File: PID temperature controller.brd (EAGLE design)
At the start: 82.2 x 72.4 mm, 12 parts, among them IC1 MAX6675

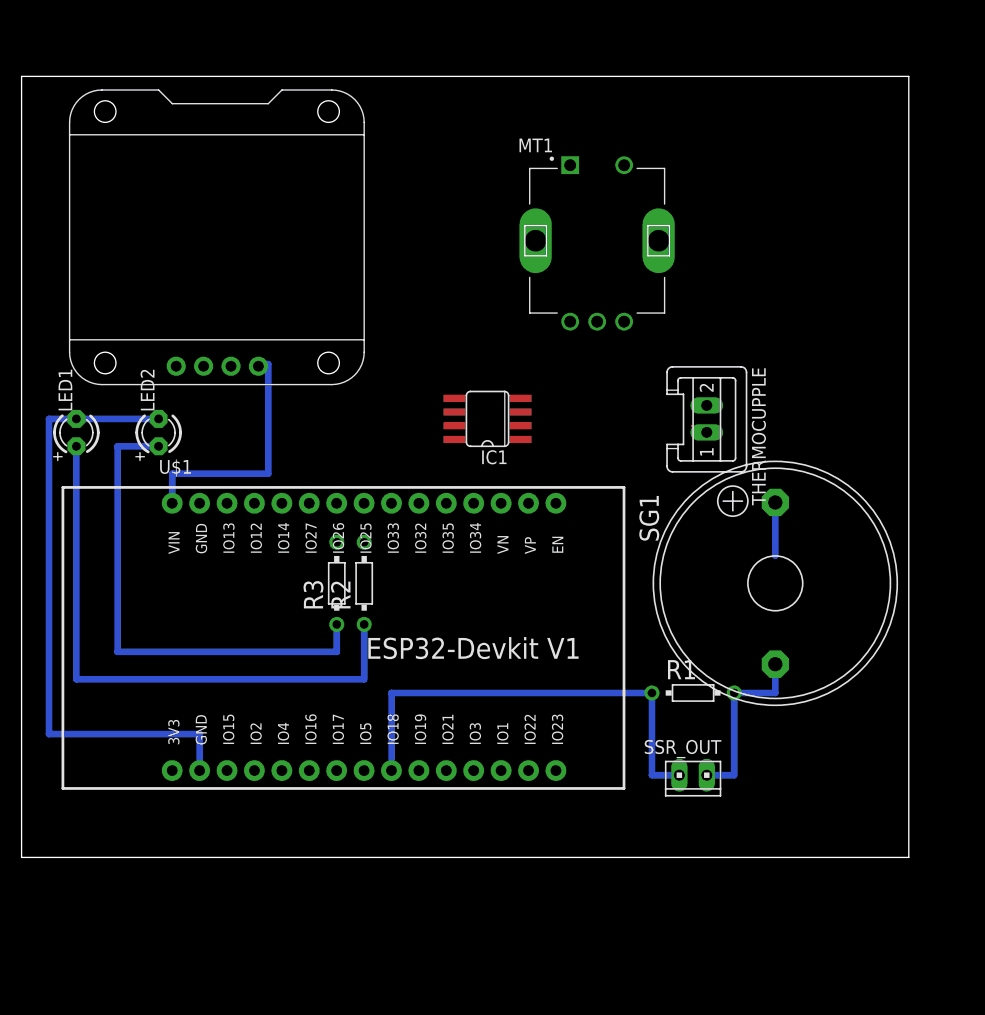
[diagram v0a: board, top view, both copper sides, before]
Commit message: Eagle Schematic and Brd file added
Eagle Schematic and Brd file added
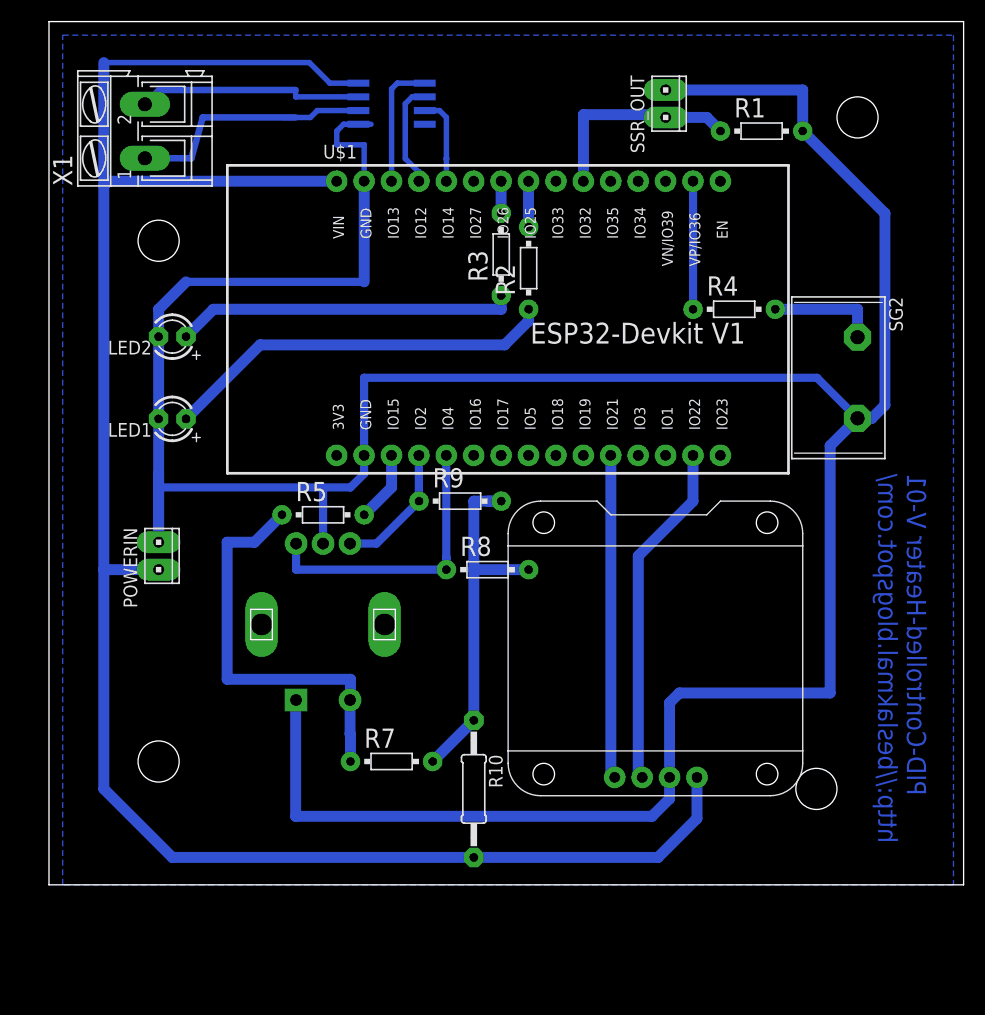
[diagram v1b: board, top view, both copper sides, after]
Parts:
- removed MT1: PEC11R-4215F-S0024, rotary encoder:XDCR_PEC11R-4215F-S0024
- removed SG1: EB2209A, buzzer:EB2209A
- removed THERMOCUPPLE: (no value), con-amp-mt:S02P
- added ENCODER: PEC11R-4215F-S0024, rotary encoder:XDCR_PEC11R-4215F-S0024
- added POWERIN: 5 V, con-amp:10X02MTA
- added R10: 0 Ohm, adafruit:0207/12
- added R4: 100 Ohm, resistor-power:RS1/8
- added R5: 0 Ohm, resistor-power:RS1/8
- added R7, R8, R9: 10k, resistor-power:RS1/8
- added SG2: B/C11S, buzzer:B/C11S
- added X1: (no value), con-ptr500:AK300/2
- IC1: device max6675:SO08 -> MAX6675:SO08
- R2, R3: value 100k -> 100 Ohm
- moved SSR_OUT 62.3 mm to (63.5, 72.4), turned to 270 degrees
- moved U$2 55.7 mm to (62.2, 21.6)
- moved R1 52.5 mm to (72.4, 69.8)
- moved R3 34.1 mm to (48.3, 58.4)
- moved R2 32.9 mm to (50.8, 57.1)
- moved IC1 30.5 mm to (38.1, 72.4), flipped to the bottom
- moved U$1 29.3 mm to (49.5, 52.1)
- moved LED1 8.98 mm to (17.8, 43.2), turned to 180 degrees
- moved LED2 8.98 mm to (17.8, 50.8), turned to 180 degrees
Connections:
- removed net N$12: MT1.B, U$1.5
- new net N$17: R4.2, SG2.1
- new net N$18: R10.1, R7.2, R8.2, R9.2
- new net N$20: ENCODER.B, R9.1, U$1.D2
- new net N$21: ENCODER.A, R8.1, U$1.D4
- net GND: now also ENCODER.1, ENCODER.COM, POWERIN.2, SG2.2, U$1.GND@1, U$1.GND@2; no longer MT1.1, MT1.COM, SG1.-, U$1.2
- net N$1: now also U$1.D14; no longer U$1.26
- net N$10: now also ENCODER.2, R5.1, R7.1; no longer MT1.2, U$1.3
- net N$11: now also R5.2, U$1.D15; no longer MT1.A, U$1.4
- net N$15: now also U$1.D26; no longer U$1.24
- net N$16: now also U$1.D25; no longer U$1.23
- net N$2: now also U$1.D12; no longer U$1.27
- net N$3: now also U$1.D13; no longer U$1.28
- net N$4: now also R4.1, U$1.D27; no longer SG1.+, U$1.24
- net N$5: now also X1.2; no longer THERMOCUPPLE.2
- net N$6: now also X1.1; no longer THERMOCUPPLE.1
- net N$7: now also U$1.D21; no longer U$1.11
- net N$8: now also U$1.D22; no longer U$1.14
- net N$9: now also U$1.D32; no longer U$1.9
- net VCC: now also POWERIN.1, R10.2, U$1.VIN; no longer U$1.30
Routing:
- net GND: track 73.4 -> 307.8 mm
- net VCC: track 22.9 -> 181.4 mm
- net N$10: track 0.00 -> 38.5 mm
- net N$18: track 0.00 -> 34.6 mm
- net N$8: track 0.00 -> 32.1 mm
- net N$7: track 0.00 -> 29.8 mm
- net N$21: track 0.00 -> 28.6 mm
- net N$6: track 1.63 -> 24.2 mm
- net N$9: track 41.9 -> 20.7 mm
- net N$5: track 0.87 -> 21.0 mm
- net N$13: track 53.3 -> 36.6 mm
- net N$14: track 45.7 -> 31.5 mm, vias 1 -> 0
- net N$20: track 0.00 -> 12.4 mm
- net N$3: track 0.00 -> 11.0 mm
- net N$17: track 0.00 -> 10.2 mm
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- added copper zone on layer 16, net GND
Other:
- board size 82.2 x 72.4 mm -> 84.8 x 80 mm
- board text added: "PID-Controlled-Heater V-01 http://beslakmal.blogspot.com/"
